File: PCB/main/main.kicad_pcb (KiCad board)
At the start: 2 copper layers, 121.9 x 91.4 mm, 63 parts, among them IC1 LM358DT, IC2 LM358DT, IC3 AT24C256C-SSHL-T, IC4 FT230XS-R, IC5 MCP73831T-2ACI_OT, IC6 MCP1700T-3302E_TT, J1 Conn_01x33_Female, J10 PZ254V-11-02P, J2 Conn_01x33_Female, J3 Conn_01x33_Female, J4 Conn_01x33_Female, J5 47346-0001, J6 PZ254V-11-02P, J7 PZ254V-11-02P, J8 MTP125-1103S1, J9 PZ254V-11-02P, Q1 IRF9540NPbF

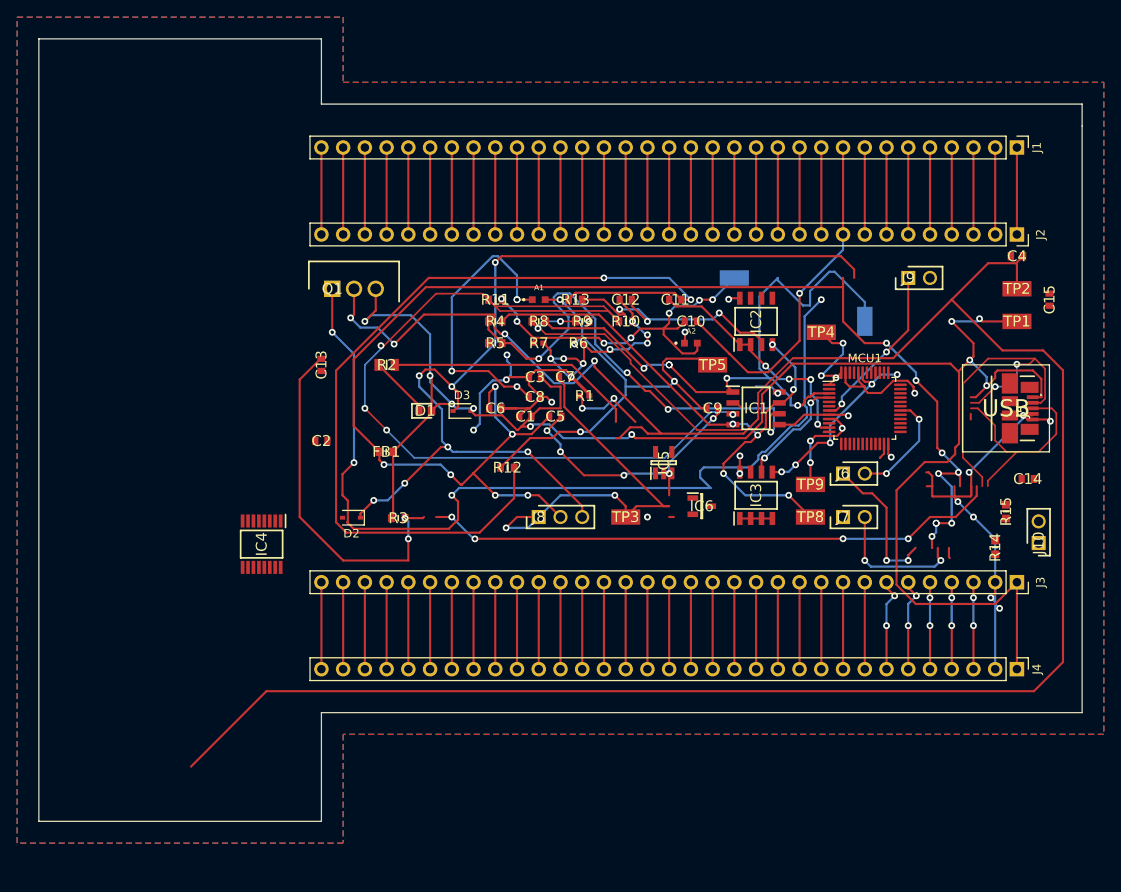
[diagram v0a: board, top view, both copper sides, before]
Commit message: new PCB
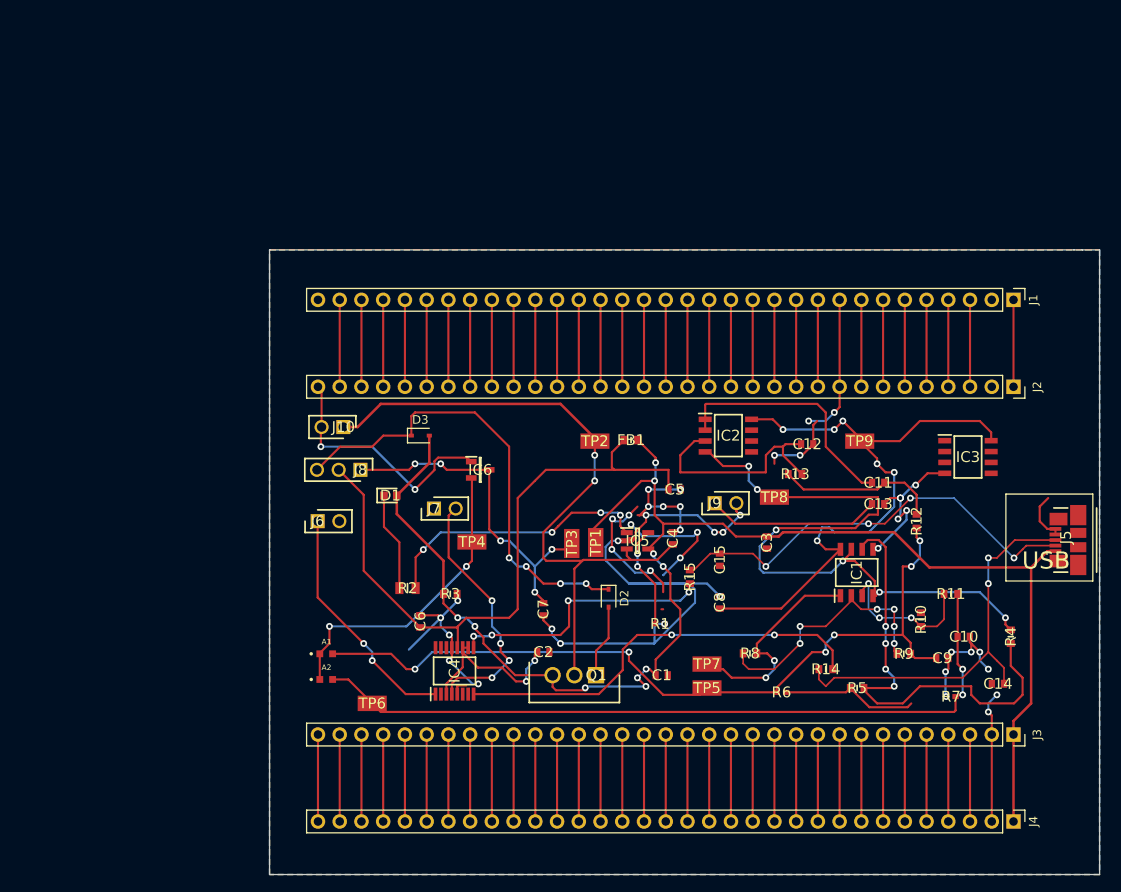
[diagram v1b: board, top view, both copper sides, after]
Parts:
- removed MCU1: STM32F030C8Tx, Package_QFP:LQFP-48_7x7mm_P0.5mm
- C13, C14, C15, C2: footprint CAP1UF:CAPC1608X90N -> SamacSys_Parts:CAPC1608X90N
- IC4: footprint SamacSys_Parts:SOP64P599X175-16N -> SamacSys_Parts_Power:SOP64P599X175-16N
- IC5: footprint SamacSys_Parts:SOT95P270X145-5N -> SamacSys_Parts_Power:SOT95P270X145-5N
- IC6: footprint SamacSys_Parts:SOT95P237X112-3N -> SamacSys_Parts_Power:SOT95P237X112-3N
- J10, J6, J7, J9: footprint SamacSys_Parts:HDRV2W64P0X254_1X2_508X250X873P -> SamacSys_Parts_Power:HDRV2W64P0X254_1X2_508X250X873P
- J5: footprint SamacSys_Parts_Power:47346-0001 -> SamacSys_Parts_Microcontroller:47346-0001
- J8: footprint SamacSys_Parts:HDRV3W64P0X254_1X3_762X250X885P -> SamacSys_Parts_Power:HDRV3W64P0X254_1X3_762X250X885P
- R14, R15: footprint R10K:RESC1608X55N -> SamacSys_Parts:RESC1608X55N
- TP1, TP2, TP3, TP4, TP5, TP8, TP9: footprint SamacSys_Parts:5017 -> SamacSys_Parts_Power:5017
- TP6, TP7: footprint SamacSys_Parts:5017 -> SamacSys_Parts_Power:5017; moved to F.Cu
- moved J10 82.4 mm to (101.6, 98.7), turned to 180 degrees
- moved R4 70.6 mm to (179.6, 123.2), turned to 90 degrees
- moved C13 67.1 mm to (164.1, 107.7), turned to 0 degrees
- moved TP6 65.3 mm to (105.0, 131.0), turned to 0 degrees
- moved R7 63.4 mm to (172.6, 130.2), turned to 180 degrees
- moved R11 63.4 mm to (172.6, 118.2)
- moved J6 61.7 mm to (98.6, 109.7)
- moved R5 58.4 mm to (161.7, 129.2)
- moved A2 58.0 mm to (99.6, 128.2)
- moved TP1 55.6 mm to (131.1, 112.2), turned to -90 degrees
- moved Q1 54.7 mm to (131.2, 127.7), turned to 180 degrees
- moved R9 54.0 mm to (167.1, 125.2)
- moved TP2 52.4 mm to (131.0, 100.3)
- moved C4 52.0 mm to (140.1, 111.7), turned to -90 degrees
- moved C15 49.1 mm to (145.6, 114.2), turned to 90 degrees
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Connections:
- net Net-(C13-Pad1) renamed /microcontroller_interfacing/NRST
- net USATR1_RX renamed /Power/PA10
- IC3 pad 5: /microcontroller_interfacing/SDA_P43 -> /microcontroller_interfacing/PB7
- IC3 pad 6: /microcontroller_interfacing/SCL_P4 -> /microcontroller_interfacing/PC15
- J6 pad 2: USART1_TX -> /Power/PA9
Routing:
- net Net-(C4-Pad2): track 271.2 -> 79.9 mm, vias 4 -> 2
- net Net-(D2-Pad2): track 109.2 -> 8.55 mm, vias 4 -> 0
- net VCC: track 165.8 -> 75.1 mm, vias 15 -> 0
- net Net-(C11-Pad2): track 106.2 -> 18.9 mm, vias 2 -> 0
- net IN1+: track 103.8 -> 17.8 mm, vias 4 -> 3
- net Net-(D2-Pad1): track 114.5 -> 54.4 mm, vias 7 -> 4
- net Net-(IC4-Pad8): track 0.00 -> 49.2 mm, vias 0 -> 2
- net Vdiff: track 73.5 -> 25.6 mm, vias 5 -> 2
- net GND: track 295.9 -> 248.9 mm, vias 29 -> 40
- net Vout2: track 43.7 -> 89.0 mm, vias 7 -> 2
- net +3v3: track 67.4 -> 110.4 mm, vias 17 -> 8
- net Vout1: track 56.5 -> 94.9 mm, vias 5 -> 6
- net (no net): track 68.1 -> 31.6 mm, vias 4 -> 7
- net +5V: track 213.8 -> 180.9 mm
- net Net-(IC4-Pad9): track 0.00 -> 31.6 mm, vias 0 -> 4
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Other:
- board size 121.9 x 91.4 mm -> 97 x 73 mm
